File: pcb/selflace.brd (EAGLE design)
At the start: 100 x 82.5 mm, 35 parts, among them IC1 78L05Z, J3 AVR_SPI_PROG_3X2NS, U1 ATMEGA328P_TQFP, Y1 16MHz

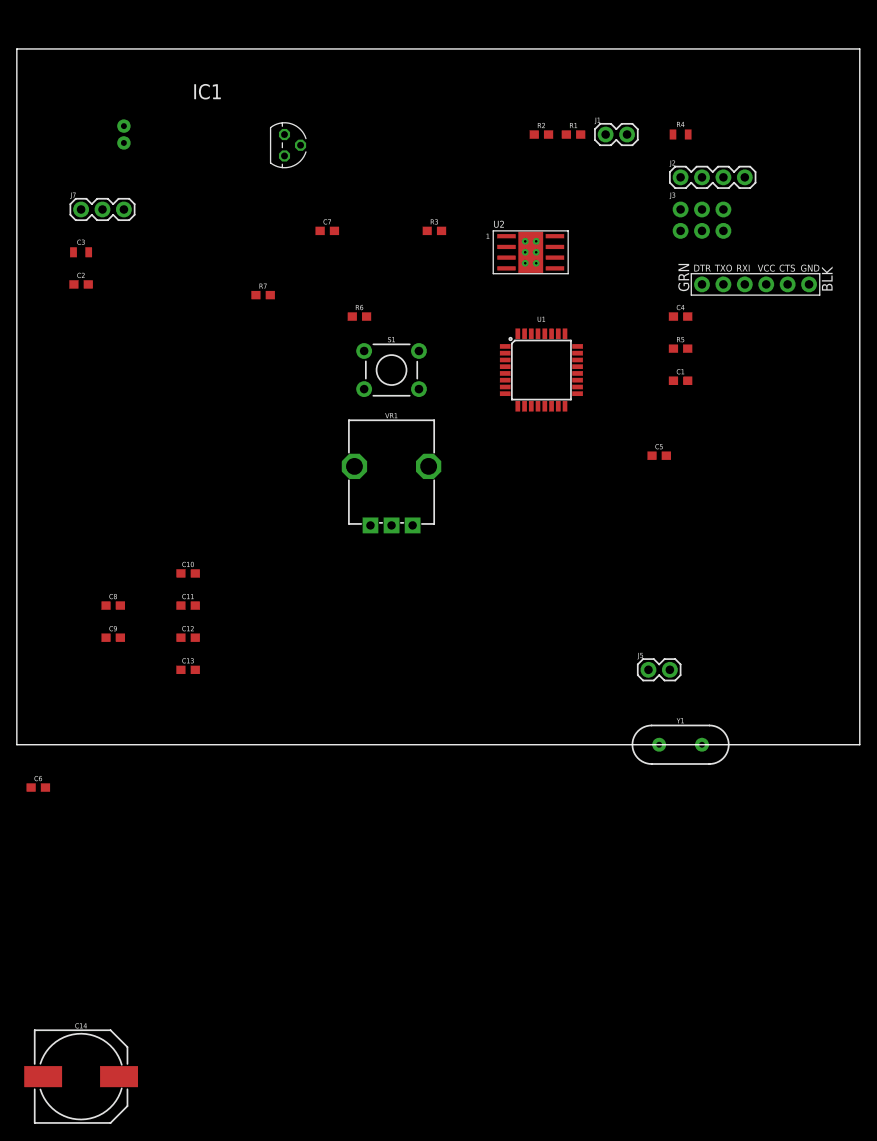
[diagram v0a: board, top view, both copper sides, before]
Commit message: nearly done! sending off for final review
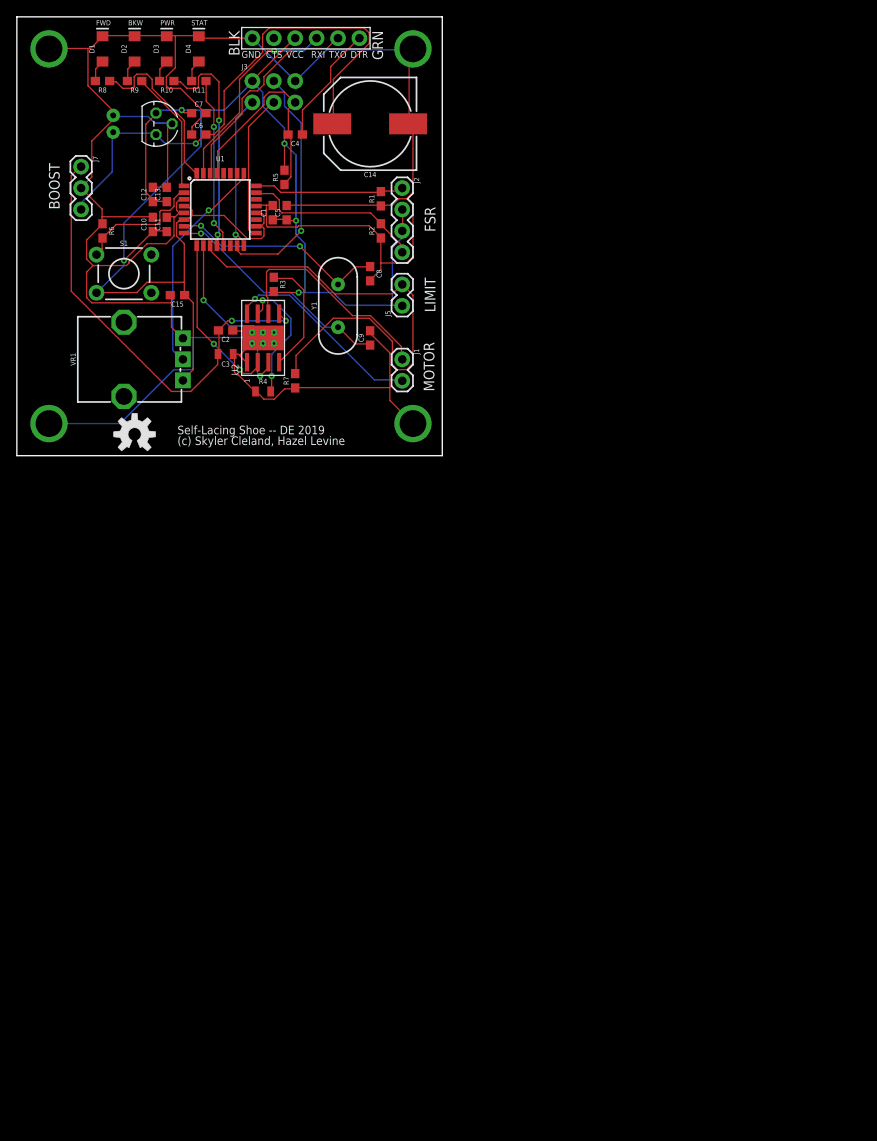
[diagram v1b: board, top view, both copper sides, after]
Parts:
- added C15: 0.1uF, SparkFun-Capacitors:0603
- added D1: FWD, SparkFun-LED:LED-1206
- added D2: BKWD, SparkFun-LED:LED-1206
- added D3: POWER, SparkFun-LED:LED-1206
- added D4: STATE, SparkFun-LED:LED-1206
- added LOGO1: OSHW-LOGOM, SparkFun-Aesthetics:OSHW-LOGO-M
- added MGT1, MGT2, MGT3, MGT4: BEAGLEBONEBLACK_MOUNTING_HOLE, BeagleBone_Black_Wireless:BEAGLEBONEBLACK_MOUNTING_HOLE
- added R10, R11, R8, R9: 220, SparkFun-Resistors:0603
- moved C14 118.1 mm to (40.6, 73.7), turned to 180 degrees
- moved C6 79.8 mm to (20.3, 72.4)
- moved Y1 66.1 mm to (36.8, 52.1), turned to 90 degrees
- moved J4 60.8 mm to (33.0, 83.8), turned to 180 degrees
- moved R4 58.2 mm to (27.9, 41.9)
- moved C13 56.4 mm to (16.5, 65.3), turned to 90 degrees
- moved J3 53.0 mm to (29.2, 77.5)
- moved C5 52.8 mm to (30.7, 63.1), turned to 90 degrees
- moved C12 52.7 mm to (14.9, 65.3), turned to 90 degrees
- moved C1 52.3 mm to (29.1, 63.1), turned to 90 degrees
- moved J5 52.1 mm to (44.5, 52.1), turned to 90 degrees
- moved R5 51.2 mm to (30.5, 67.3), turned to 90 degrees
- moved C4 50.6 mm to (31.8, 72.4), turned to 180 degrees
- moved C8 49.8 mm to (40.6, 55.9), turned to 270 degrees
- moved C9 46.8 mm to (40.6, 48.3), turned to 90 degrees
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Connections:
- new net DIG2: R8.1, U1.32
- new net DIG3: R9.1, U1.1
- new net DIG8: R10.1, U1.12
- new net DIG9: R11.1, U1.13
- new net N$13: D1.A, R8.2
- new net N$14: D2.A, R9.2
- new net N$15: D3.A, R10.2
- new net N$16: D4.A, R11.2
- net GND: now also C15.2, D1.C, D2.C, D3.C, D4.C, MGT1.P$1, MGT2.P$1, MGT3.P$1, MGT4.P$1
- net VCC: now also C15.1
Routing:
- net GND: track 0.00 -> 309.1 mm
- net VCC: track 0.00 -> 179.3 mm, vias 0 -> 5
- net N$12: track 0.00 -> 63.8 mm, vias 0 -> 1
- net N$2: track 0.00 -> 58.2 mm
- net VCC_1: track 0.00 -> 52.7 mm, vias 0 -> 2
- net MOSI: track 0.00 -> 28.6 mm, vias 0 -> 1
- net N$11: track 0.00 -> 27.6 mm, vias 0 -> 1
- net DIG8: track 0.00 -> 27.1 mm, vias 0 -> 2
- net N$4: track 0.00 -> 26.6 mm
- net RESET: track 0.00 -> 26.4 mm
- net N$6: track 0.00 -> 26.3 mm, vias 0 -> 1
- net N$7: track 0.00 -> 25.9 mm, vias 0 -> 2
- net RX: track 0.00 -> 25.4 mm
- net TX: track 0.00 -> 24.1 mm, vias 0 -> 1
- net N$5: track 0.00 -> 24.0 mm, vias 0 -> 1
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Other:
- board size 100 x 82.5 mm -> 50.5 x 52.1 mm
- board text added: "(c) Skyler Cleland, Hazel Levine"
- board text added: "BKW"
- board text added: "BOOST"
- board text added: "FSR"
- board text added: "FWD"
- board text added: "LIMIT"
- board text added: "MOTOR"
- board text added: "PWR"
- board text added: "STAT"
- board text added: "Self-Lacing Shoe -- DE 2019"
